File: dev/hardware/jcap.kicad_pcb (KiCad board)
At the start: 2 copper layers, 149.1 x 77 mm, 74 parts, among them J201 CPU PGMR, J202 GPU PGMR, J203 SPARE GPU HDR, J204 SPARE CPU HDR, J301 DC IN, J502 VGA OUT, J601 CONTROLS, SW201 CPU ~{RES}, SW202 GPU ~{RES}, SW203 DEBUG, SW601 TILT, U101 P8X32A-D40, U201 P8X32A-D40, U302 LF33_TO220, U401 24LC256, U402 24LC256, U601 74HC165, U602 74HC165, Y101 6.5MHz, Y201 6.5MHz

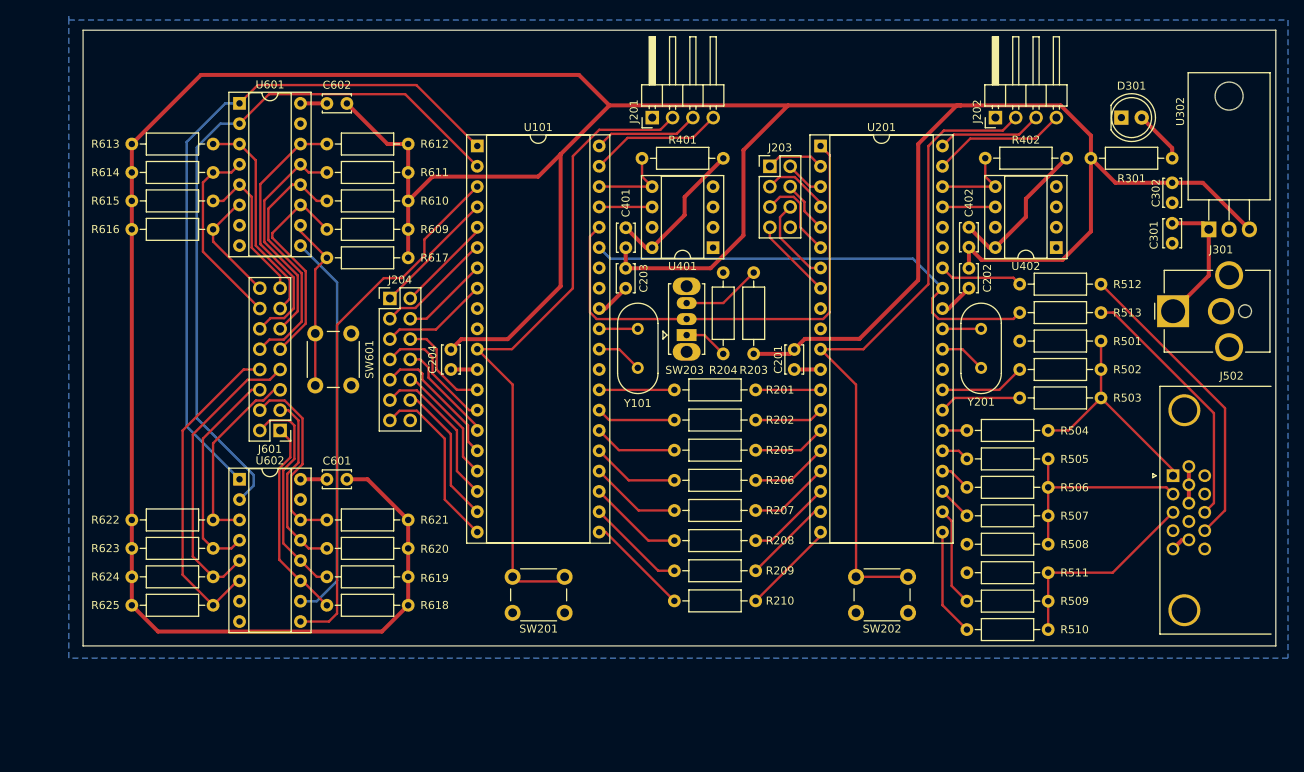
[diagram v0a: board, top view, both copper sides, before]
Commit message: Nearly final PCB
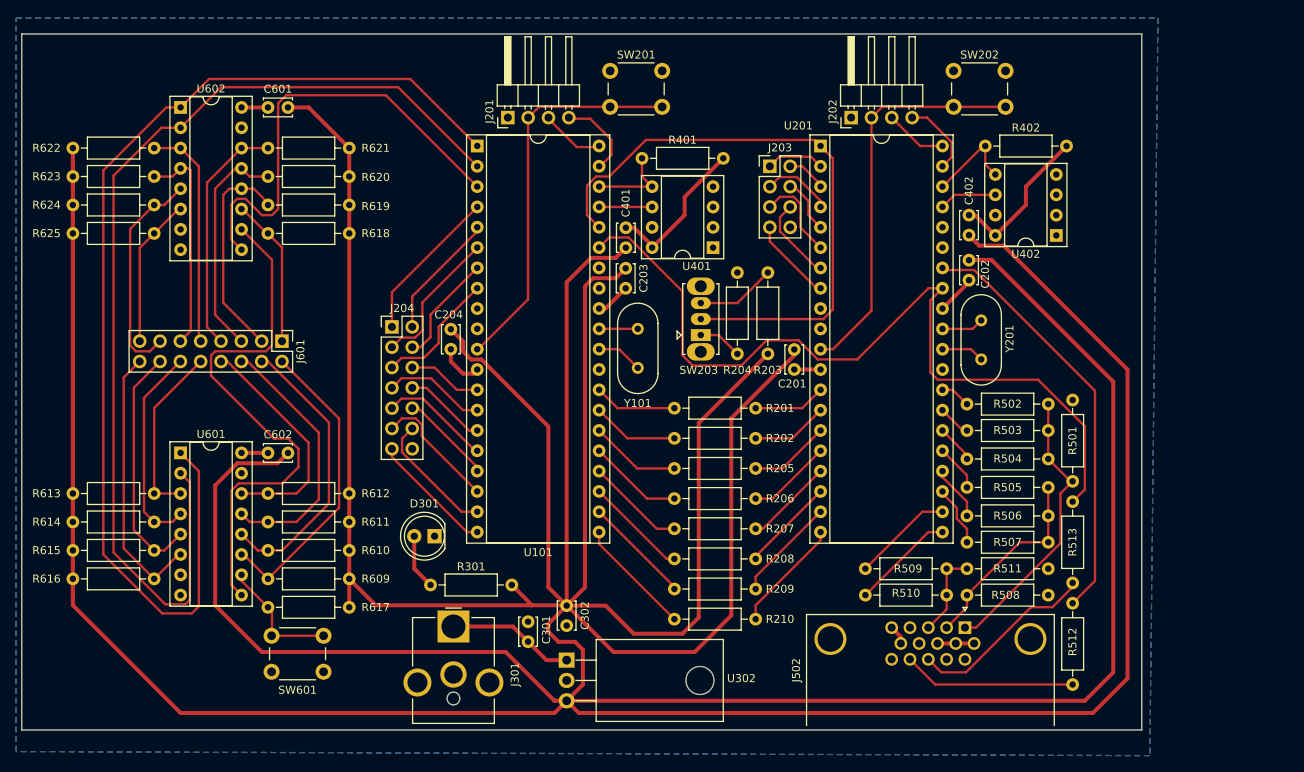
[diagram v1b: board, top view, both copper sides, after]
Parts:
- moved D301 100.5 mm to (133.6, 128.8), turned to 180 degrees
- moved J301 98.2 mm to (136.0, 140.1), turned to 0 degrees
- moved U302 96.7 mm to (150.1, 144.3), turned to -90 degrees
- moved C301 93.4 mm to (145.3, 139.5), turned to -90 degrees
- moved C302 92.3 mm to (150.1, 140.0)
- moved R301 89.9 mm to (143.3, 134.9), turned to 180 degrees
- moved SW201 68.0 mm to (155.6, 70.6), turned to 0 degrees
- moved SW202 68.0 mm to (198.5, 70.6), turned to 0 degrees
- moved R512 50.2 mm to (213.4, 147.3), turned to 90 degrees
- moved C601 47.1 mm to (112.8, 75.2)
- moved R619 47.1 mm to (112.8, 87.4)
- moved R620 47.1 mm to (112.8, 83.8)
- moved R621 47.1 mm to (112.8, 80.3)
- moved R622 47.1 mm to (98.6, 80.3)
- moved R623 47.1 mm to (98.6, 83.8)
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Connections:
- J601 pad 10: /Input/IN10 -> /Input/IN13
- J601 pad 11: /Input/IN11 -> /Input/IN6
- J601 pad 12: /Input/IN12 -> /Input/IN14
- J601 pad 13: /Input/IN13 -> /Input/IN7
- J601 pad 14: /Input/IN14 -> /Input/IN15
- J601 pad 15: /Input/IN15 -> /Input/IN8
- J601 pad 2: /Input/IN2 -> /Input/IN9
- J601 pad 3: /Input/IN3 -> /Input/IN2
- J601 pad 4: /Input/IN4 -> /Input/IN10
- J601 pad 5: /Input/IN5 -> /Input/IN3
- J601 pad 6: /Input/IN6 -> /Input/IN11
- J601 pad 7: /Input/IN7 -> /Input/IN4
- J601 pad 8: /Input/IN8 -> /Input/IN12
- J601 pad 9: /Input/IN9 -> /Input/IN5
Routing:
- net +3.3V: track 471.3 -> 838.7 mm
- net ~{INPUTS_PL}: track 87.3 -> 138.4 mm
- net V_SYNC: track 60.2 -> 104.0 mm
- net H_SYNC: track 10.5 -> 53.1 mm
- net INPUTS_CLK: track 89.3 -> 130.0 mm
- net /Propellers/~{SER_RES_CPU}: track 83.4 -> 48.9 mm
- net /Propellers/~{SER_RES_GPU}: track 83.3 -> 49.8 mm
- net /Input/IN8: track 40.8 -> 18.8 mm
- net /Input/IN16: track 14.3 -> 34.1 mm
- net /Input/SHIFT_IN: track 49.4 -> 66.9 mm
- net Net-(J502-Pad14): track 38.3 -> 21.9 mm
- net /VGA_DAC/BLUE_OUT: track 25.9 -> 10.9 mm
- net /Propellers/DEBUG: track 63.1 -> 75.9 mm
- net /Input/IN9: track 27.1 -> 38.4 mm
- net /Input/IN15: track 19.2 -> 30.2 mm
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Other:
- board size 149.1 x 77 mm -> 140 x 87 mm
